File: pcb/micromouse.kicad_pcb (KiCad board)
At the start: 2 copper layers, 46 x 75.9 mm, 59 parts, among them J1 PINHD_1x6_Female, J10 B2B-PH-K-S, J11 B2B-PH-K-S, J12 PINHD_1x6_Female, J13 B6B-ZR, J14 PINHD_1x5_Male, J15 PINHD_1x5_Male, J16 PINHD_1x2_Male, J2 PINHD_1x6_Female, J3 PINHD_1x4_Female, J4 PINHD_1x6_Female, J5 PINHD_1x4_Female, J6 PINHD_1x5_Female, J7 PINHD_1x5_Female, J8 PINHD_1x2_Female, J9 B6B-ZR, M1 Left, M2 Right, SW1 SW_DIP_x04, U1 STM32F411RETx, U2 ICM-42688-P, U3 L293DD, U4 AZ1117-3.3, Y1 32.768 kHz 7 pF, Y2 25 MHz 10 pF

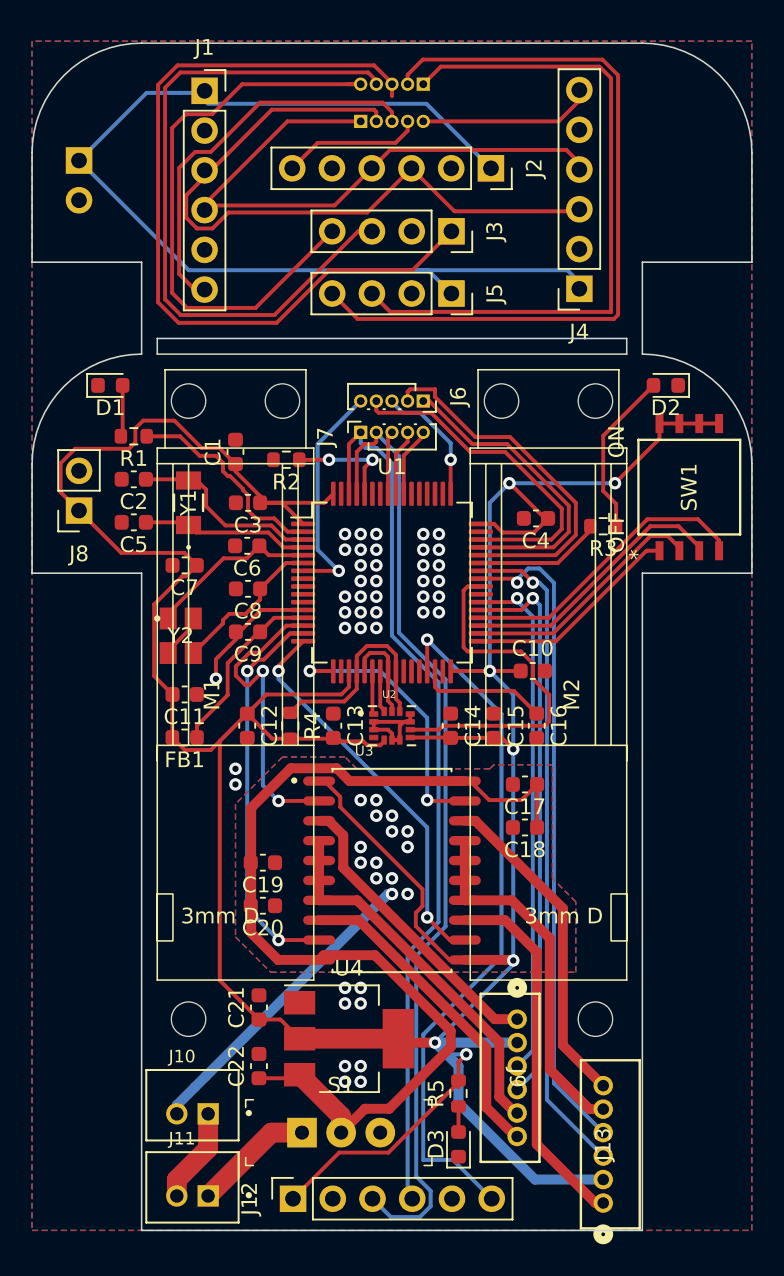
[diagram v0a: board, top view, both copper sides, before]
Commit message: Add files via upload
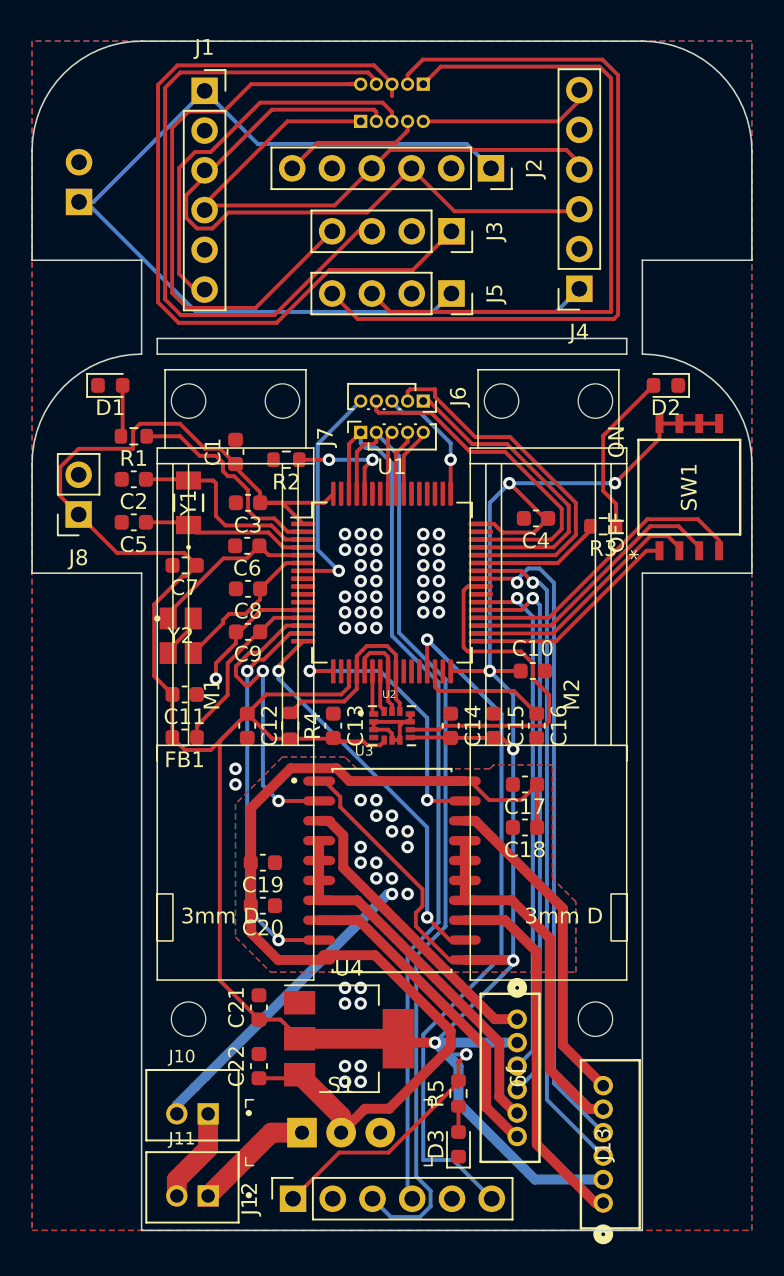
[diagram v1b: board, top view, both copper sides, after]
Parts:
- moved J16 2.65 mm to (127.0, 75.8), turned to 0 degrees
- moved J8 0.25 mm to (127.0, 95.8)
- moved NT1 0.25 mm to (136.2, 104.8)
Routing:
- net /Breakout Board/+3.3V: track 69.5 -> 71.1 mm
- net Net-(U3-PC14): track 11.6 -> 12.2 mm
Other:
- board size 46 x 75.9 mm -> 46 x 76 mm
